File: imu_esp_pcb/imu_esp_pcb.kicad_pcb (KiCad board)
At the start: 2 copper layers, 19 parts, among them J3 Conn_01x02_Pin, U1 MPU-6050, U2 ESP32-C3-WROOM-02, U3 PTS647SM38SMTR2LFS, U4 XC6206P332MR-G, U5 1N5819HW-7-F

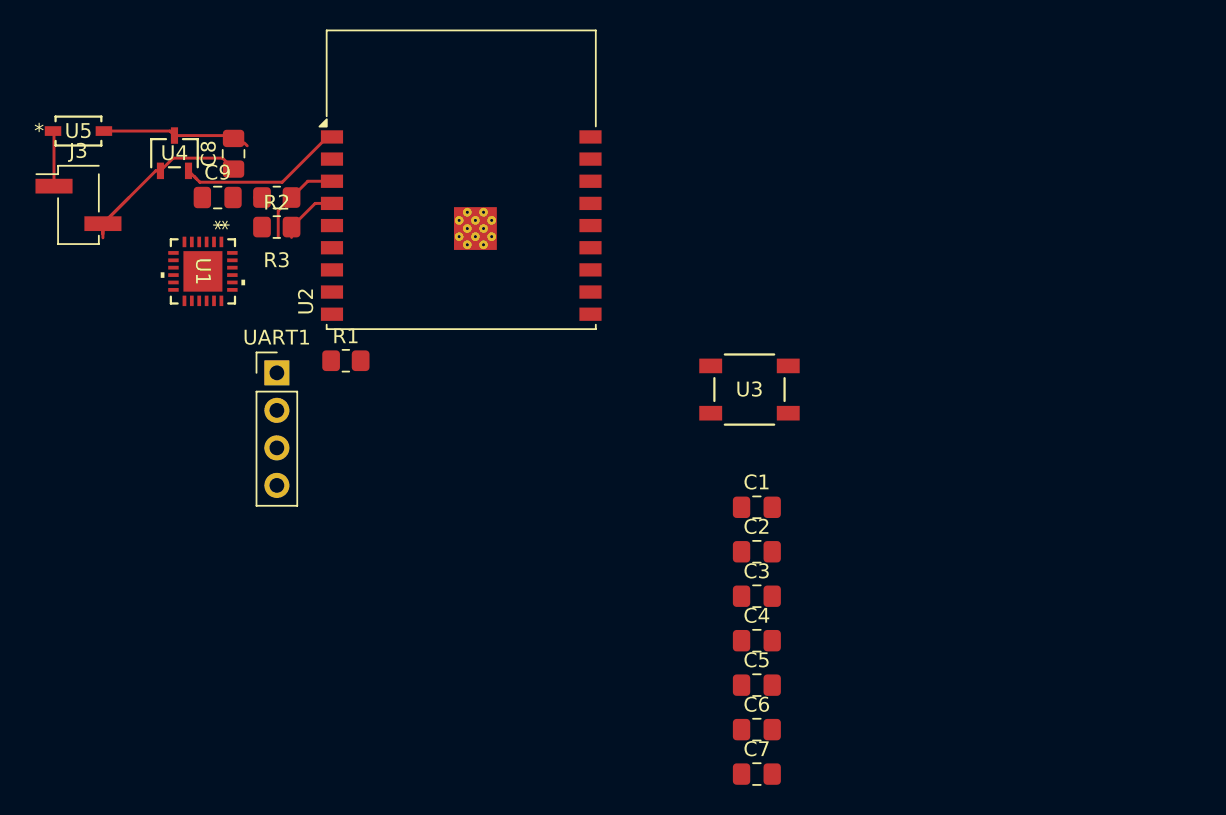
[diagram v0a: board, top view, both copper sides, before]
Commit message: Updated PCB design
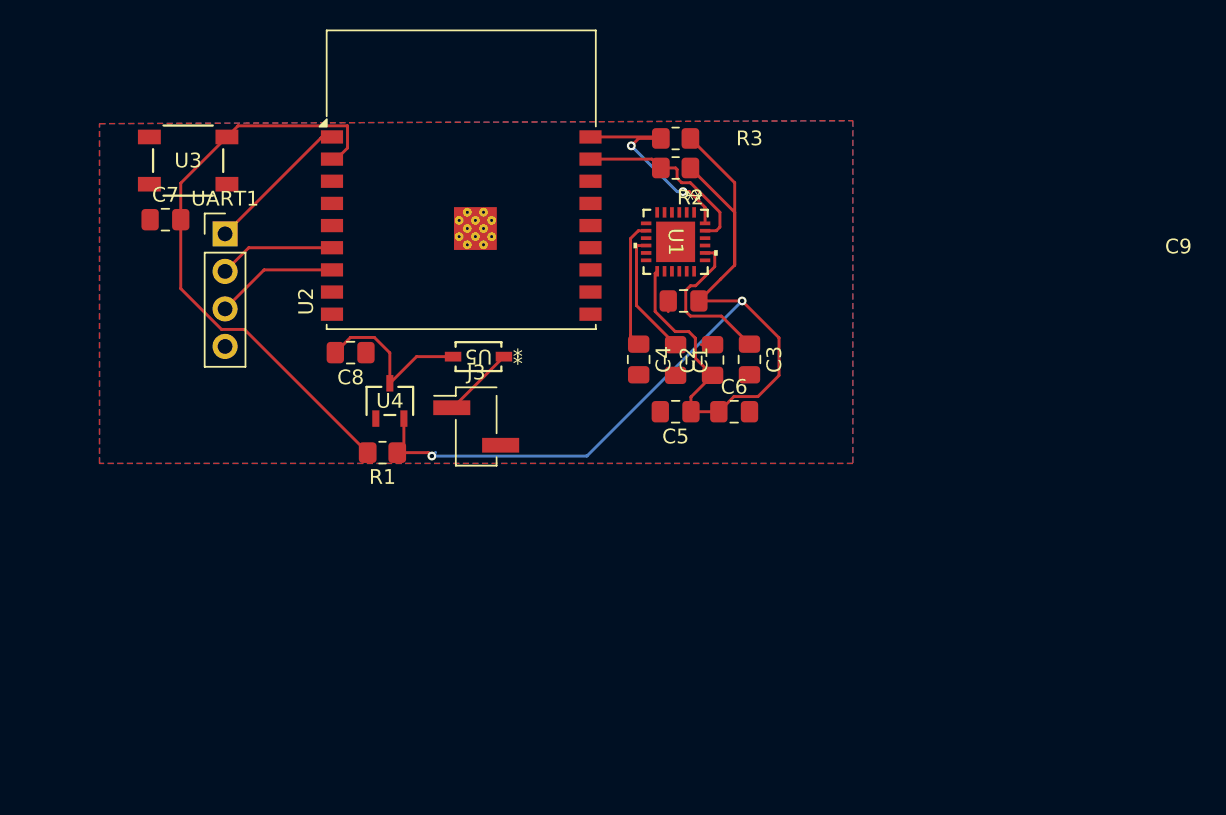
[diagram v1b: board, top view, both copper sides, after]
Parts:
- moved C7 54.9 mm to (62.5, 75.0)
- moved U3 41.0 mm to (64.0, 71.0)
- moved C9 32.3 mm to (97.5, 80.5)
- moved U1 32.1 mm to (97.0, 76.5)
- moved U5 31.1 mm to (83.7, 84.3), turned to 180 degrees
- moved J3 30.8 mm to (83.5, 89.0)
- moved R2 27.3 mm to (97.0, 71.5), turned to 180 degrees
- moved R3 27.3 mm to (97.0, 69.5), turned to 0 degrees
- moved U4 22.2 mm to (77.7, 87.3)
- moved C6 21.6 mm to (101.0, 88.0)
- moved C4 20.7 mm to (94.5, 84.5), turned to -90 degrees
- moved C5 19.3 mm to (97.0, 88.0), turned to 180 degrees
- moved C3 16.0 mm to (102.0, 84.5), turned to -90 degrees
- moved C8 15.6 mm to (75.0, 84.0), turned to 180 degrees
- moved C2 13.3 mm to (99.5, 84.5), turned to 90 degrees
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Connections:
- U2 pad 17: unconnected-(U2-IO1-Pad17) -> SCL
- U2 pad 18: unconnected-(U2-IO0-Pad18) -> SDA
- U2 pad 3: SDA -> unconnected-(U2-IO4-Pad3)
- U2 pad 4: SCL -> unconnected-(U2-IO5-Pad4)
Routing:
- net +3.3V: track 12.0 -> 90.9 mm, vias 0 -> 2
- net RESET: track 0.00 -> 40.2 mm
- net GND: track 15.2 -> 2.65 mm
- net Net-(U1-CPOUT): track 0.00 -> 10.8 mm
- net Net-(U1-VLOGIC): track 0.00 -> 8.65 mm
- net SCL: track 4.10 -> 12.7 mm
- net SDA: track 6.25 -> 14.8 mm, vias 0 -> 2
- net Net-(U1-REGOUT): track 0.00 -> 8.42 mm
- net Net-(U2-IO8): track 0.00 -> 8.33 mm
- net Net-(U2-IO7): track 0.00 -> 7.90 mm
- net Net-(U4-VIN): track 8.99 -> 11.6 mm
- net Net-(J3-Pin_1): track 3.76 -> 4.96 mm
- added copper zone on B.Cu, net GND
- added copper zone on F.Cu, net GND
